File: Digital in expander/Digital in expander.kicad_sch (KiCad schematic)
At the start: 60 parts, among them J1 Screw_Terminal_01x02, J10 Screw_Terminal_01x02, J11 Screw_Terminal_01x02, J12 Screw_Terminal_01x02, J13 Screw_Terminal_01x02, J14 Screw_Terminal_01x02, J15 Screw_Terminal_01x02, J16 Screw_Terminal_01x02, J17 Conn_01x04_Pin, J18 Conn_01x04_Pin, J19 Conn_01x04_Pin, J2 Screw_Terminal_01x02, J20 Conn_01x04_Pin, J21 Conn_01x04_Pin, J22 Conn_01x03_Pin, J3 Screw_Terminal_01x02, J4 Screw_Terminal_01x02, J5 Screw_Terminal_01x02, J6 Screw_Terminal_01x02, J7 Screw_Terminal_01x02, J8 Screw_Terminal_01x02, J9 Screw_Terminal_01x02, U1 PC847, U2 PC847, U3 PC847, U4 PC847, U5 MCP23017_SO

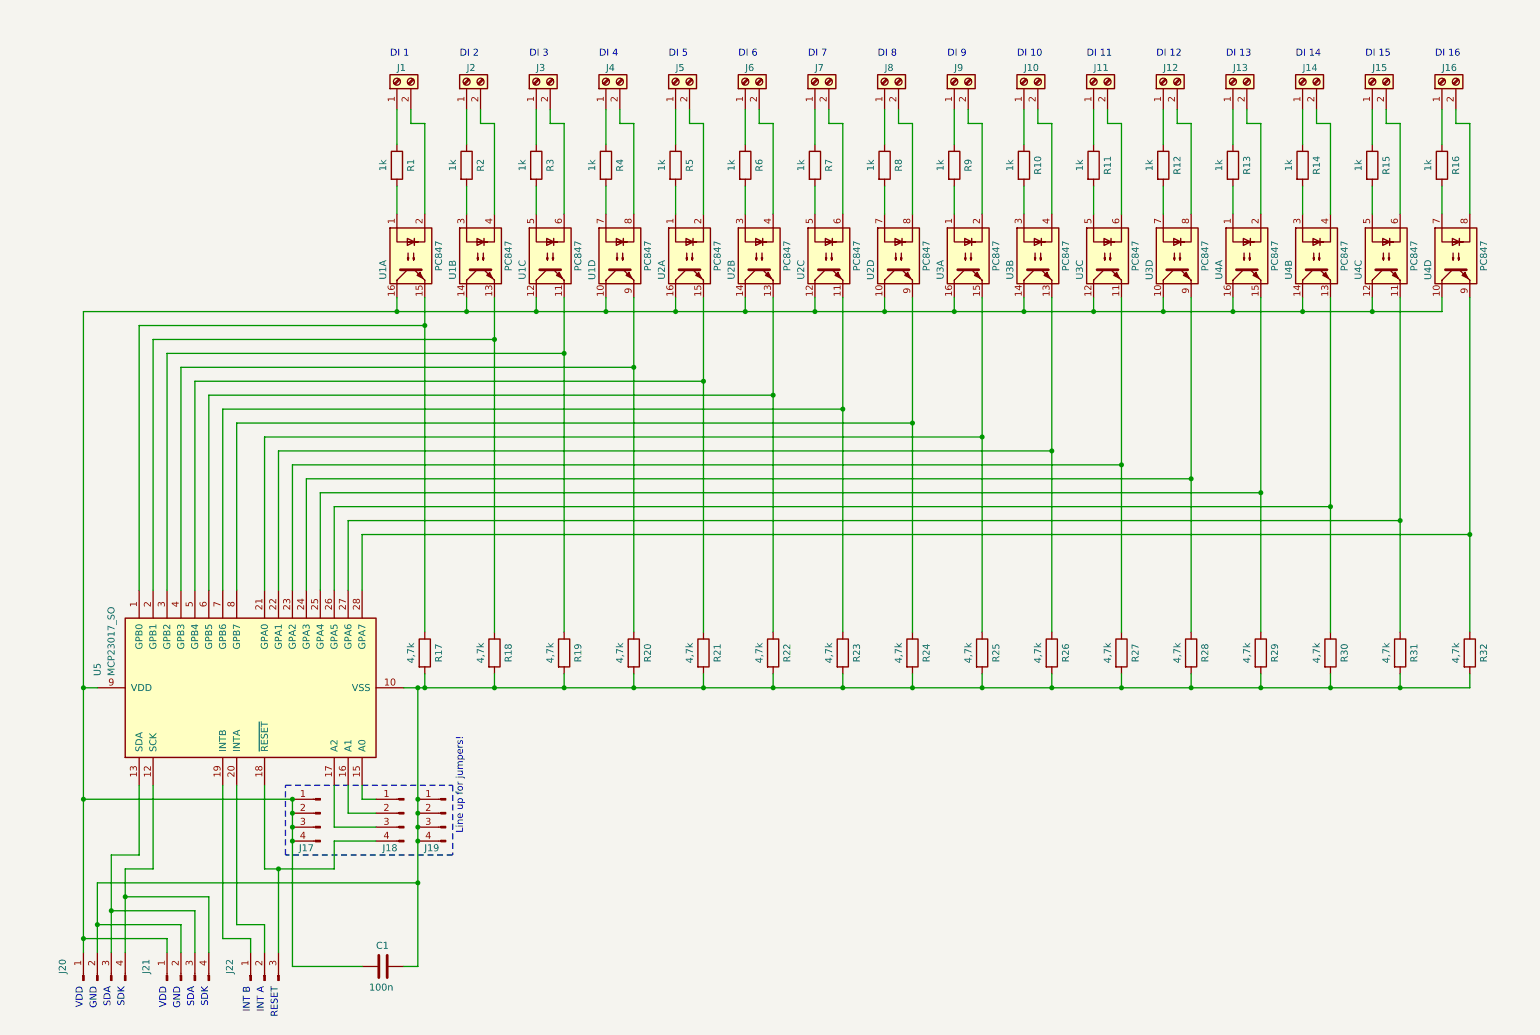
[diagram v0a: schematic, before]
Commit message: Nu borde det fungera bättre
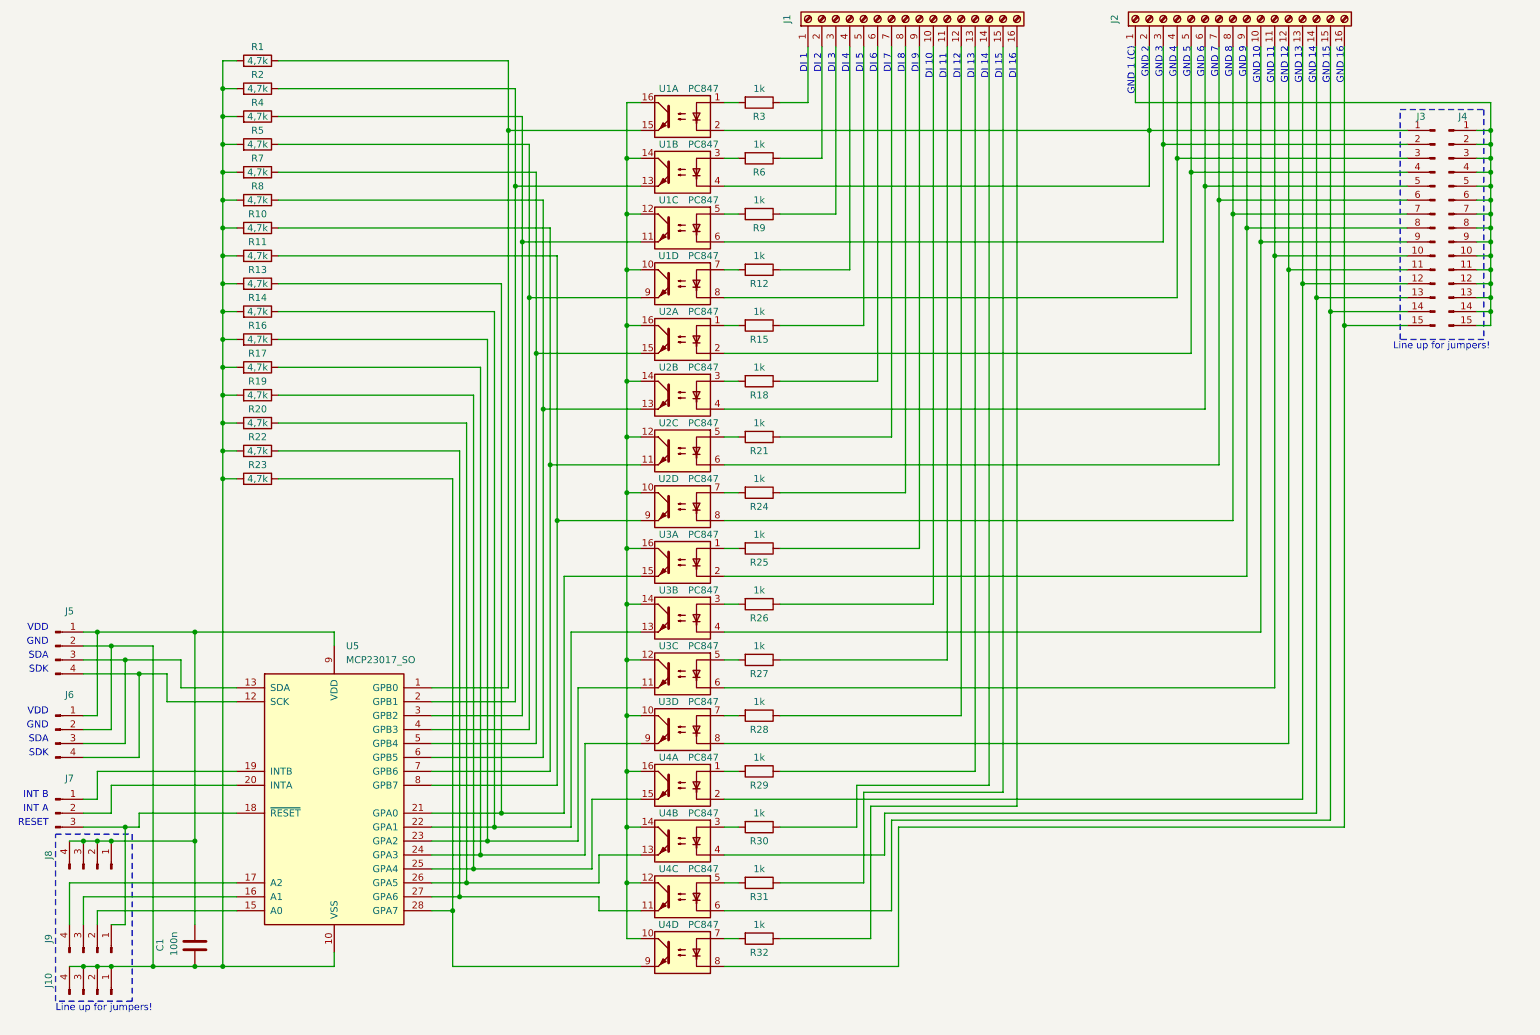
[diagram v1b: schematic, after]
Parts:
- removed J1, J10, J11, J12, J13, J14, J15, J16, J2, J3, J4, J5, J6, J7, J8, J9: Screw_Terminal_01x02, symbol Connector:Screw_Terminal_01x02
- removed R18, R21, R24, R25, R26, R27, R28, R29, R30, R31, R32: 4,7k, symbol Device:R
- added J1, J2: Screw_Terminal_01x16, symbol Connector:Screw_Terminal_01x16
- added J3, J4: Conn_01x15_Pin, symbol Connector:Conn_01x15_Pin
- added R1, R10, R11, R13, R14, R16, R2, R4, R5, R7, R8: 4,7k, symbol Device:R
- renumbered J19 to J10, J20 to J5, J21 to J6, J22 to J7, J17 to J8, J18 to J9, R4 to R12, R5 to R15, R6 to R18, R7 to R21, R8 to R24, R9 to R25, R10 to R26, R11 to R27, R12 to R28, R13 to R29, R1 to R3, R14 to R30, R15 to R31, R16 to R32, R2 to R6, R3 to R9
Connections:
- net at U1.15, U5.1 (GPB0): now also R1.1; no longer R17.1
- net at C1.2, J10.1 (Pin_1), J10.2 (Pin_2)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: now also R1.2, R10.2, R11.2, R13.2, R14.2, R16.2, R2.2, R4.2, R5.2, R7.2, R8.2
- net at U2.15, U5.5 (GPB4): now also R7.1
- net at R15.1: now also J1.5 (Pin_5)
- net at U1.10, U1.12, U1.14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: no longer C1.1, J5.1 (Pin_1), J6.1 (Pin_1), J8.1 (Pin_1), J8.2 (Pin_2), J8.3 (Pin_3), J8.4 (Pin_4), U5.9 (VDD)
- net at R26.1: now also J1.10 (Pin_10)
- net at U4.15, U5.25 (GPA4): now also R19.1
- net at U4.2: now also J2.13 (Pin_13), J3.12 (Pin_12)
- net at R32.1: now also J1.16 (Pin_16)
- net at U4.8: now also J2.16 (Pin_16), J3.15 (Pin_15)
- net at U4.9, U5.28 (GPA7): now also R23.1
- net at R30.1: now also J1.14 (Pin_14)
- net at U4.4: now also J2.14 (Pin_14), J3.13 (Pin_13)
- net at U5.15 (A0): now also J9.2 (Pin_2); no longer J9.1 (Pin_1)
- net at U5.16 (A1): now also J9.3 (Pin_3); no longer J9.2 (Pin_2)
- net at U5.17 (A2): now also J9.4 (Pin_4); no longer J9.3 (Pin_3)
- net at J7.3 (Pin_3), U5.18 (~{RESET}): now also J9.1 (Pin_1); no longer J9.4 (Pin_4)
- net at U1.13, U5.2 (GPB1): now also R2.1
- net at U3.15, U5.21 (GPA0): now also R13.1
- net at U3.13, U5.22 (GPA1): now also R14.1
- net at U3.11, U5.23 (GPA2): now also R16.1
- net at U3.9, U5.24 (GPA3): now also R17.1
- net at U4.13, U5.26 (GPA5): now also R20.1
- net at U4.11, U5.27 (GPA6): now also R22.1
- net at U1.11, U5.3 (GPB2): now also R4.1; no longer R19.1
- net at U1.9, U5.4 (GPB3): now also R5.1; no longer R20.1
- net at U2.13, U5.6 (GPB5): now also R8.1; no longer R22.1
- net at U2.11, U5.7 (GPB6): now also R10.1; no longer R23.1
- net at U2.9, U5.8 (GPB7): now also R11.1
- net at R3.1: now also J1.1 (Pin_1)
- net at R25.1: now also J1.9 (Pin_9)
- net at R28.1: now also J1.12 (Pin_12)
- net at R27.1: now also J1.11 (Pin_11)
- net at U3.6: now also J2.11 (Pin_11), J3.10 (Pin_10)
- net at R24.1: now also J1.8 (Pin_8)
- net at R9.1: now also J1.3 (Pin_3)
- net at U1.6: now also J2.3 (Pin_3), J3.2 (Pin_2)
- net at U3.4: now also J2.10 (Pin_10), J3.9 (Pin_9)
- net at U2.8: now also J2.8 (Pin_8), J3.7 (Pin_7)
- net at U2.2: now also J2.5 (Pin_5), J3.4 (Pin_4)
- net at R29.1: now also J1.13 (Pin_13)
- net at U1.2: now also U1.4, J2.2 (Pin_2), J3.1 (Pin_1)
- net at R21.1: now also J1.7 (Pin_7)
- net at U2.6: now also J2.7 (Pin_7), J3.6 (Pin_6)
- net at R6.1: now also J1.2 (Pin_2)
- net at R12.1: now also J1.4 (Pin_4)
- net at U1.8: now also J2.4 (Pin_4), J3.3 (Pin_3)
- net at U2.4: now also J2.6 (Pin_6), J3.5 (Pin_5)
- net at U4.6: now also J2.15 (Pin_15), J3.14 (Pin_14)
- net at U3.8: now also J2.12 (Pin_12), J3.11 (Pin_11)
- net at U3.2: now also J2.9 (Pin_9), J3.8 (Pin_8)
- net at R18.1: now also J1.6 (Pin_6)
- net at R31.1: now also J1.15 (Pin_15)
- new net: J2.1 (Pin_1), J4.1 (Pin_1), J4.10 (Pin_10), J4.11 (Pin_11), J4.12 (Pin_12), J4.13 (Pin_13), J4.14 (Pin_14), J4.15 (Pin_15), J4.2 (Pin_2), J4.3 (Pin_3), J4.4 (Pin_4), J4.5 (Pin_5), J4.6 (Pin_6), J4.7 (Pin_7), J4.8 (Pin_8), J4.9 (Pin_9)
- new net: C1.1, J5.1 (Pin_1), J6.1 (Pin_1), J8.1 (Pin_1), J8.2 (Pin_2), J8.3 (Pin_3), J8.4 (Pin_4), U5.9 (VDD)
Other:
- note added: "GND 1 (C)"
- note added: "GND 10"
- note added: "GND 11"
- note added: "GND 12"
- note added: "GND 13"
- note added: "GND 14"
- note added: "GND 15"
- note added: "GND 16"
- note added: "GND 2"
- note added: "GND 3"
- note added: "GND 4"
- note added: "GND 5"
- note added: "GND 6"
- note added: "GND 7"
- note added: "GND 8"
- note added: "GND 9"
- moved on the sheet: C1, J10, J5, J6, J7, J8, J9, R12, R15, R18, R21, R24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

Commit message: Förbättrad läsbarhet
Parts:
- R1, R10, R11, R13, R14, R16, R2, R4, R5, R7, R8: value 4,7k -> 1k
- R18, R21, R24, R25, R26, R27, R28, R29, R30, R31, R32: value 1k -> 4,7k
- renumbered J7 to J10, J8 to J5, J9 to J6, J10 to J7, J5 to J8, J6 to J9
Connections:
- net at J4.1 (Pin_1), J4.10 (Pin_10), J4.11 (Pin_11)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: now also J1.1 (Pin_1), U1.2; no longer J2.1 (Pin_1)
- net at J3.9 (Pin_9), U3.4: now also J1.10 (Pin_10); no longer J2.10 (Pin_10)
- net at J3.10 (Pin_10), U3.6: now also J1.11 (Pin_11); no longer J2.11 (Pin_11)
- net at J3.11 (Pin_11), U3.8: now also J1.12 (Pin_12); no longer J2.12 (Pin_12)
- net at J3.12 (Pin_12), U4.2: now also J1.13 (Pin_13); no longer J2.13 (Pin_13)
- net at J3.13 (Pin_13), U4.4: now also J1.14 (Pin_14); no longer J2.14 (Pin_14)
- net at J3.14 (Pin_14), U4.6: now also J1.15 (Pin_15); no longer J2.15 (Pin_15)
- net at J3.15 (Pin_15), U4.8: now also J1.16 (Pin_16); no longer J2.16 (Pin_16)
- net at J3.1 (Pin_1), U1.4: now also J1.2 (Pin_2); no longer J2.2 (Pin_2), U1.2
- net at J3.2 (Pin_2), U1.6: now also J1.3 (Pin_3); no longer J2.3 (Pin_3)
- net at J3.3 (Pin_3), U1.8: now also J1.4 (Pin_4); no longer J2.4 (Pin_4)
- net at J3.4 (Pin_4), U2.2: now also J1.5 (Pin_5); no longer J2.5 (Pin_5)
- net at J3.5 (Pin_5), U2.4: now also J1.6 (Pin_6); no longer J2.6 (Pin_6)
- net at J3.6 (Pin_6), U2.6: now also J1.7 (Pin_7); no longer J2.7 (Pin_7)
- net at J3.7 (Pin_7), U2.8: now also J1.8 (Pin_8); no longer J2.8 (Pin_8)
- net at J3.8 (Pin_8), U3.2: now also J1.9 (Pin_9); no longer J2.9 (Pin_9)
- net at R15.1: now also J2.15 (Pin_15); no longer J1.5 (Pin_5)
- net at R15.2: now also U4.5; no longer U2.1
- net at C1.1, J5.1 (Pin_1), J5.2 (Pin_2)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: now also U1.10, U1.12, U1.14, U1.16, U2.10, U2.12, U2.14, U2.16, U3.10, U3.12, U3.14, U3.16, U4.10, U4.12, U4.14, U4.16
- net at C1.2, J7.1 (Pin_1), J7.2 (Pin_2)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: now also R18.2, R21.2, R24.2, R25.2, R26.2, R27.2, R28.2, R29.2, R30.2, R31.2, R32.2; no longer R1.2, R10.2, R11.2, R13.2, R14.2, R16.2, R2.2, R4.2, R5.2, R7.2, R8.2
- net at R26.1: now also U3.13, U5.22 (GPA1); no longer J1.10 (Pin_10)
- net at U3.3: now also R10.2; no longer R26.2
- net at U3.15, U5.21 (GPA0): now also R25.1; no longer R13.1
- net at U4.1: now also R13.2; no longer R29.2
- net at U4.15, U5.25 (GPA4): now also R29.1; no longer R19.1
- net at U2.11, U5.7 (GPB6): now also R23.1; no longer R10.1
- net at U1.15, U5.1 (GPB0): now also R17.1; no longer R1.1
- net at U5.15 (A0): now also J6.1 (Pin_1); no longer J6.2 (Pin_2)
- net at U5.16 (A1): now also J6.2 (Pin_2); no longer J6.3 (Pin_3)
- net at U5.17 (A2): now also J6.3 (Pin_3); no longer J6.4 (Pin_4)
- net at J10.3 (Pin_3), U5.18 (~{RESET}): now also J6.4 (Pin_4); no longer J6.1 (Pin_1)
- net at U1.13, U5.2 (GPB1): now also R18.1; no longer R2.1
- net at U3.11, U5.23 (GPA2): now also R27.1; no longer R16.1
- net at U3.9, U5.24 (GPA3): now also R28.1; no longer R17.1
- net at U4.13, U5.26 (GPA5): now also R30.1; no longer R20.1
- net at U4.11, U5.27 (GPA6): now also R31.1; no longer R22.1
- net at U4.9, U5.28 (GPA7): no longer R23.1
- net at U1.11, U5.3 (GPB2): now also R19.1; no longer R4.1
- net at U1.9, U5.4 (GPB3): now also R20.1; no longer R5.1
- net at U2.15, U5.5 (GPB4): now also R21.1; no longer R7.1
- net at U2.13, U5.6 (GPB5): now also R22.1; no longer R8.1
- net at U2.9, U5.8 (GPB7): now also R24.1; no longer R11.1
- net at R3.1: now also J2.3 (Pin_3); no longer J1.1 (Pin_1)
- net at U1.1: now also R1.2; no longer R3.2
- net at U3.1: now also R9.2; no longer R25.2
- net at U3.7: now also R12.2; no longer R28.2
- net at U2.7: now also R8.2; no longer R24.2
- net at R6.1: now also J2.6 (Pin_6); no longer J1.2 (Pin_2)
- net at R6.2: now also U2.3; no longer U1.3
- net at R32.1: no longer J1.16 (Pin_16)
- net at R9.1: now also J2.9 (Pin_9); no longer J1.3 (Pin_3)
- net at R12.1: now also J2.12 (Pin_12); no longer J1.4 (Pin_4)
- net at U4.3: now also R14.2; no longer R30.2
- net at U4.7: now also R16.2; no longer R32.2
- net at U2.5: now also R7.2; no longer R21.2
- net at U3.5: now also R11.2; no longer R27.2
- net at U1.7: now also R4.2; no longer R12.2
- net at U1.5: now also R3.2; no longer R9.2
- new net: J2.10 (Pin_10), R10.1
- new net: J2.5 (Pin_5), R5.1
- new net: R5.2, U2.1
- new net: R2.2, U1.3
- new net: J2.8 (Pin_8), R8.1
- new net: J2.1 (Pin_1), R1.1
- new net: J2.13 (Pin_13), R13.1
- new net: J2.16 (Pin_16), R16.1
- new net: J2.2 (Pin_2), R2.1
- new net: J2.7 (Pin_7), R7.1
- new net: J2.14 (Pin_14), R14.1
- new net: J2.11 (Pin_11), R11.1
- new net: J2.4 (Pin_4), R4.1
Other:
- moved on the sheet: J10, J5, J6, J7, J8, J9
